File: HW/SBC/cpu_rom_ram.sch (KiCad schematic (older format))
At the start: 6 parts, among them U1 WD65C02_, U2 28C256, U3 AS6C62256A

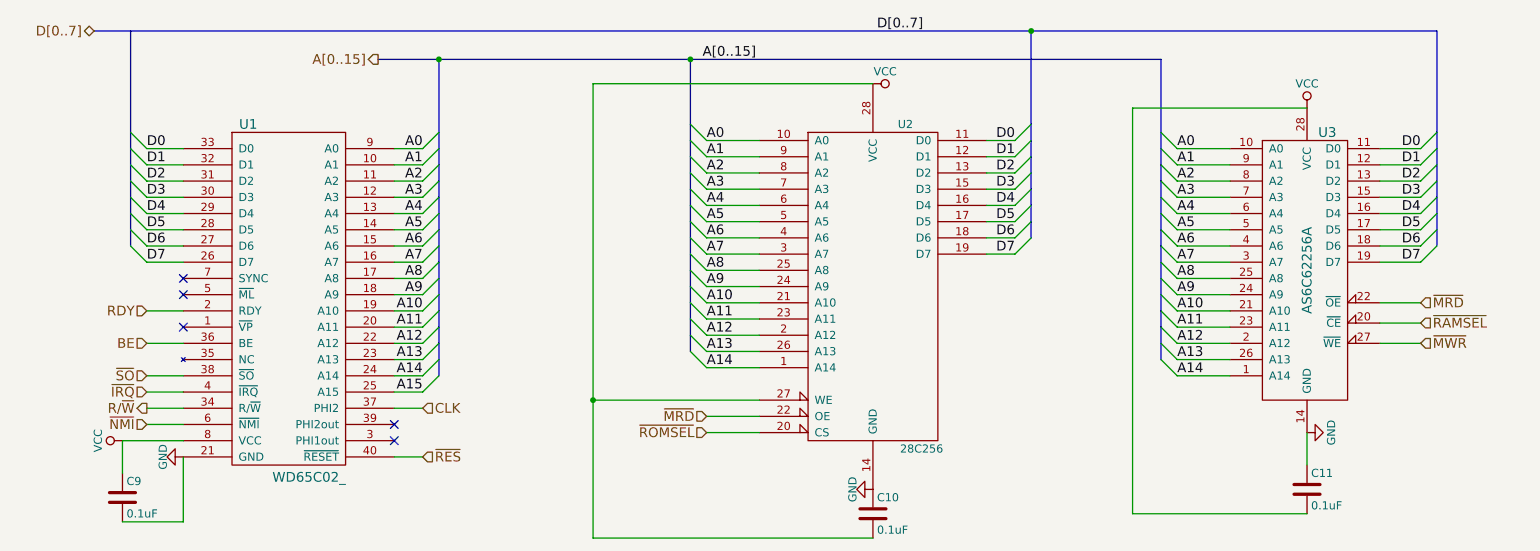
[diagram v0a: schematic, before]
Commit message: Small changes to comments.
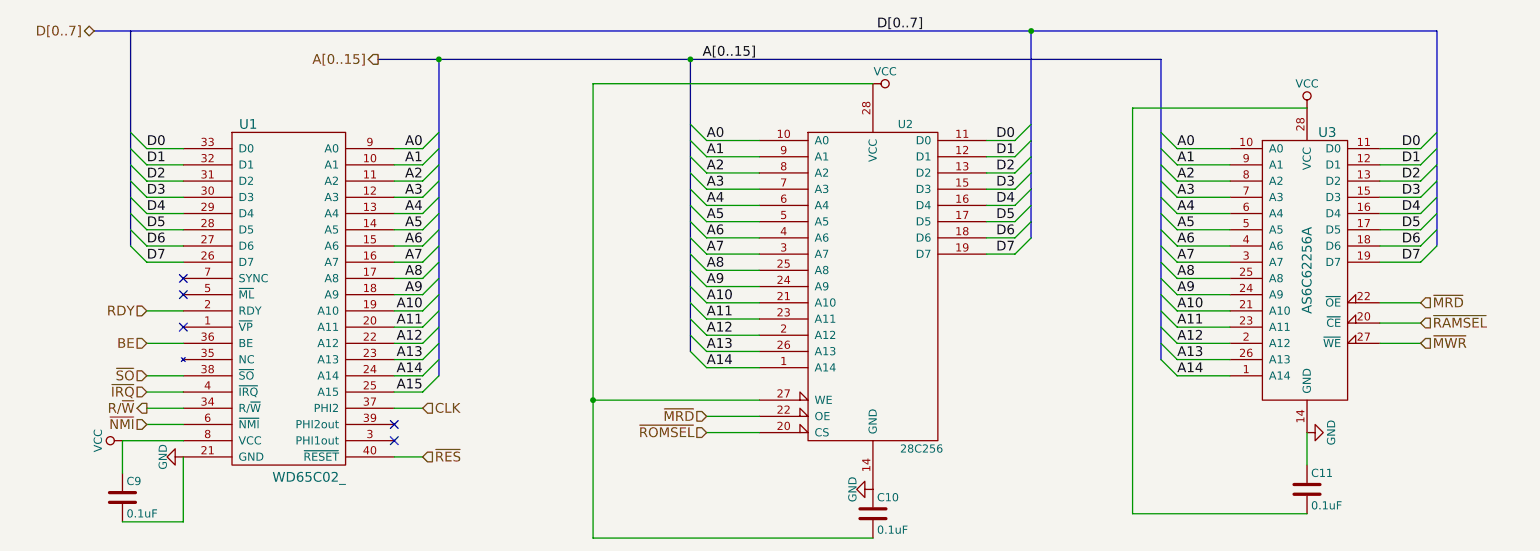
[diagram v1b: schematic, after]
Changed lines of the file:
@@
 	4050 3850 5775 3850
 Wire Wire Line
-	4050 1050 4050 3000
-Wire Wire Line
-	4050 3000 4050 3850
+	4050 1050 4050 3850
 Wire Wire Line
 	4050 1050 5775 1050
@@
 Connection ~ 4050 3000
 Wire Bus Line
-	3100 900  3100 1350
+	3100 900  3100 2850
 Wire Bus Line
-	3100 1350 3100 1450
+	4650 900  4650 2700
 Wire Bus Line
-	3100 1450 3100 1550
+	7550 900  7550 2750
 Wire Bus Line
-	3100 1550 3100 1650
+	1200 725  1200 2050
 Wire Bus Line
-	3100 1650 3100 1750
+	6750 725  6750 2000
 Wire Bus Line
-	3100 1750 3100 1850
+	9250 725  9250 2050
 Wire Bus Line
-	3100 1850 3100 1950
-Wire Bus Line
-	3100 1950 3100 2050
-Wire Bus Line
-	3100 2050 3100 2150
-Wire Bus Line
-	3100 2150 3100 2250
-Wire Bus Line
-	3100 2250 3100 2350
-Wire Bus Line
-	3100 2350 3100 2450
-Wire Bus Line
-	3100 2450 3100 2550
-Wire Bus Line
-	3100 2550 3100 2650
-Wire Bus Line
-	3100 2650 3100 2750
-Wire Bus Line
-	3100 2750 3100 2850
-Wire Bus Line
-	4650 900  4650 1300
-Wire Bus Line
-	4650 1300 4650 1400
-Wire Bus Line
-	4650 1400 4650 1500
-Wire Bus Line
-	4650 1500 4650 1600
-Wire Bus Line
-	4650 1600 4650 1700
-Wire Bus Line
-	4650 1700 4650 1800
-Wire Bus Line
-	4650 1800 4650 1900
-Wire Bus Line
-	4650 1900 4650 2000
-Wire Bus Line
-	4650 2000 4650 2100
-Wire Bus Line
-	4650 2100 4650 2200
-Wire Bus Line
-	4650 2200 4650 2300
-Wire Bus Line
-	4650 2300 4650 2400
-Wire Bus Line
-	4650 2400 4650 2500
-Wire Bus Line
-	4650 2500 4650 2600
-Wire Bus Line
-	4650 2600 4650 2700
-Wire Bus Line
-	7550 900  7550 1350
-Wire Bus Line
-	7550 1350 7550 1450
-Wire Bus Line
-	7550 1450 7550 1550
-Wire Bus Line
-	7550 1550 7550 1650
-Wire Bus Line
-	7550 1650 7550 1750
-Wire Bus Line
-	7550 1750 7550 1850
-Wire Bus Line
-	7550 1850 7550 1950
-Wire Bus Line
-	7550 1950 7550 2050
-Wire Bus Line
-	7550 2050 7550 2150
-Wire Bus Line
-	7550 2150 7550 2250
-Wire Bus Line
-	7550 2250 7550 2350
-Wire Bus Line
-	7550 2350 7550 2450
-Wire Bus Line
-	7550 2450 7550 2550
-Wire Bus Line
-	7550 2550 7550 2650
-Wire Bus Line
-	7550 2650 7550 2750
-Wire Bus Line
-	1200 725  1200 1350
-Wire Bus Line
-	1200 1350 1200 1450
-Wire Bus Line
-	1200 1450 1200 1550
-Wire Bus Line
-	1200 1550 1200 1650
-Wire Bus Line
-	1200 1650 1200 1750
-Wire Bus Line
-	1200 1750 1200 1850
-Wire Bus Line
-	1200 1850 1200 1950
-Wire Bus Line
-	1200 1950 1200 2050
-Wire Bus Line
-	6750 725  6750 1300
-Wire Bus Line
-	6750 1300 6750 1400
-Wire Bus Line
-	6750 1400 6750 1500
-Wire Bus Line
-	6750 1500 6750 1600
-Wire Bus Line
-	6750 1600 6750 1700
-Wire Bus Line
-	6750 1700 6750 1800
-Wire Bus Line
-	6750 1800 6750 1900
-Wire Bus Line
-	6750 1900 6750 2000
-Wire Bus Line
-	9250 725  9250 1350
-Wire Bus Line
-	9250 1350 9250 1450
-Wire Bus Line
-	9250 1450 9250 1550
-Wire Bus Line
-	9250 1550 9250 1650
-Wire Bus Line
-	9250 1650 9250 1750
-Wire Bus Line
-	9250 1750 9250 1850
-Wire Bus Line
-	9250 1850 9250 1950
-Wire Bus Line
-	9250 1950 9250 2050
-Wire Bus Line
-	975  725  6750 725
-Wire Bus Line
-	6750 725  9250 725
+	975  725  9250 725
 Text HLabel 975  725  0    60   BiDi ~ 0
 D[0..7]
 Wire Bus Line
-	2725 900  3100 900
-Wire Bus Line
-	3100 900  4650 900
-Wire Bus Line
-	4650 900  7550 900
+	2725 900  7550 900
 Connection ~ 6750 725
 Connection ~ 4650 900
